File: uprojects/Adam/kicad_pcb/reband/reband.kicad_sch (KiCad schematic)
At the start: 3 parts, among them U1 ESP32-C3FH4, U2 LMV324MT, U3 MAX30009ENA+T

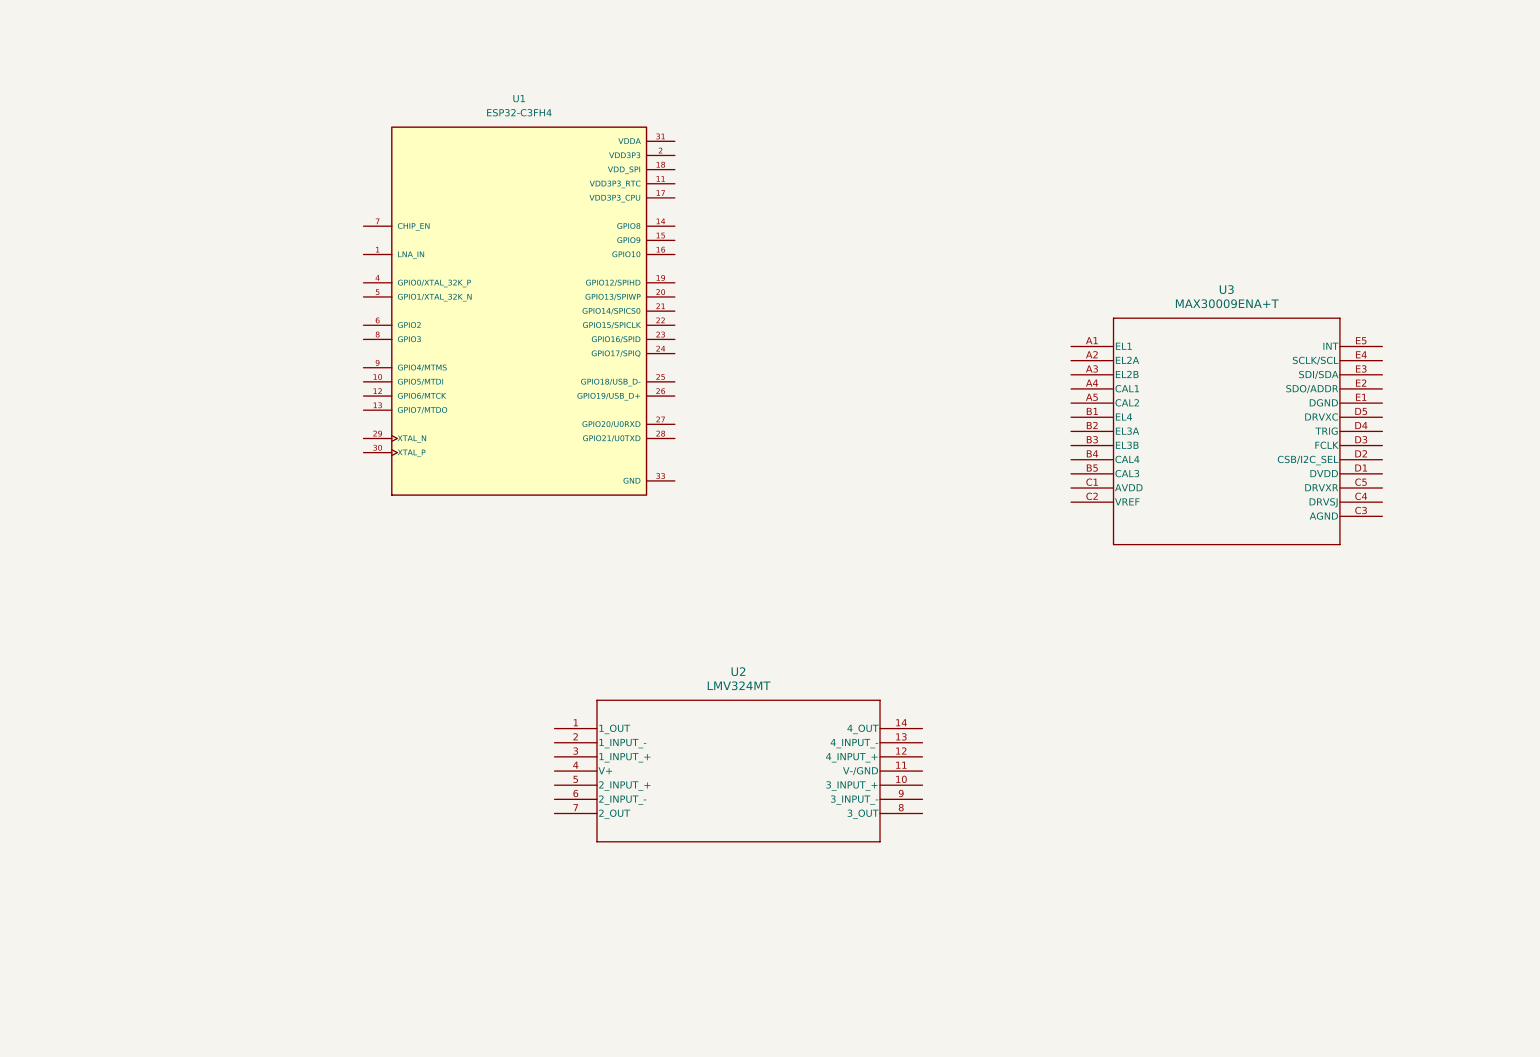
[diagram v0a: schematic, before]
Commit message: ROOM 25 MAY 2026 Updates
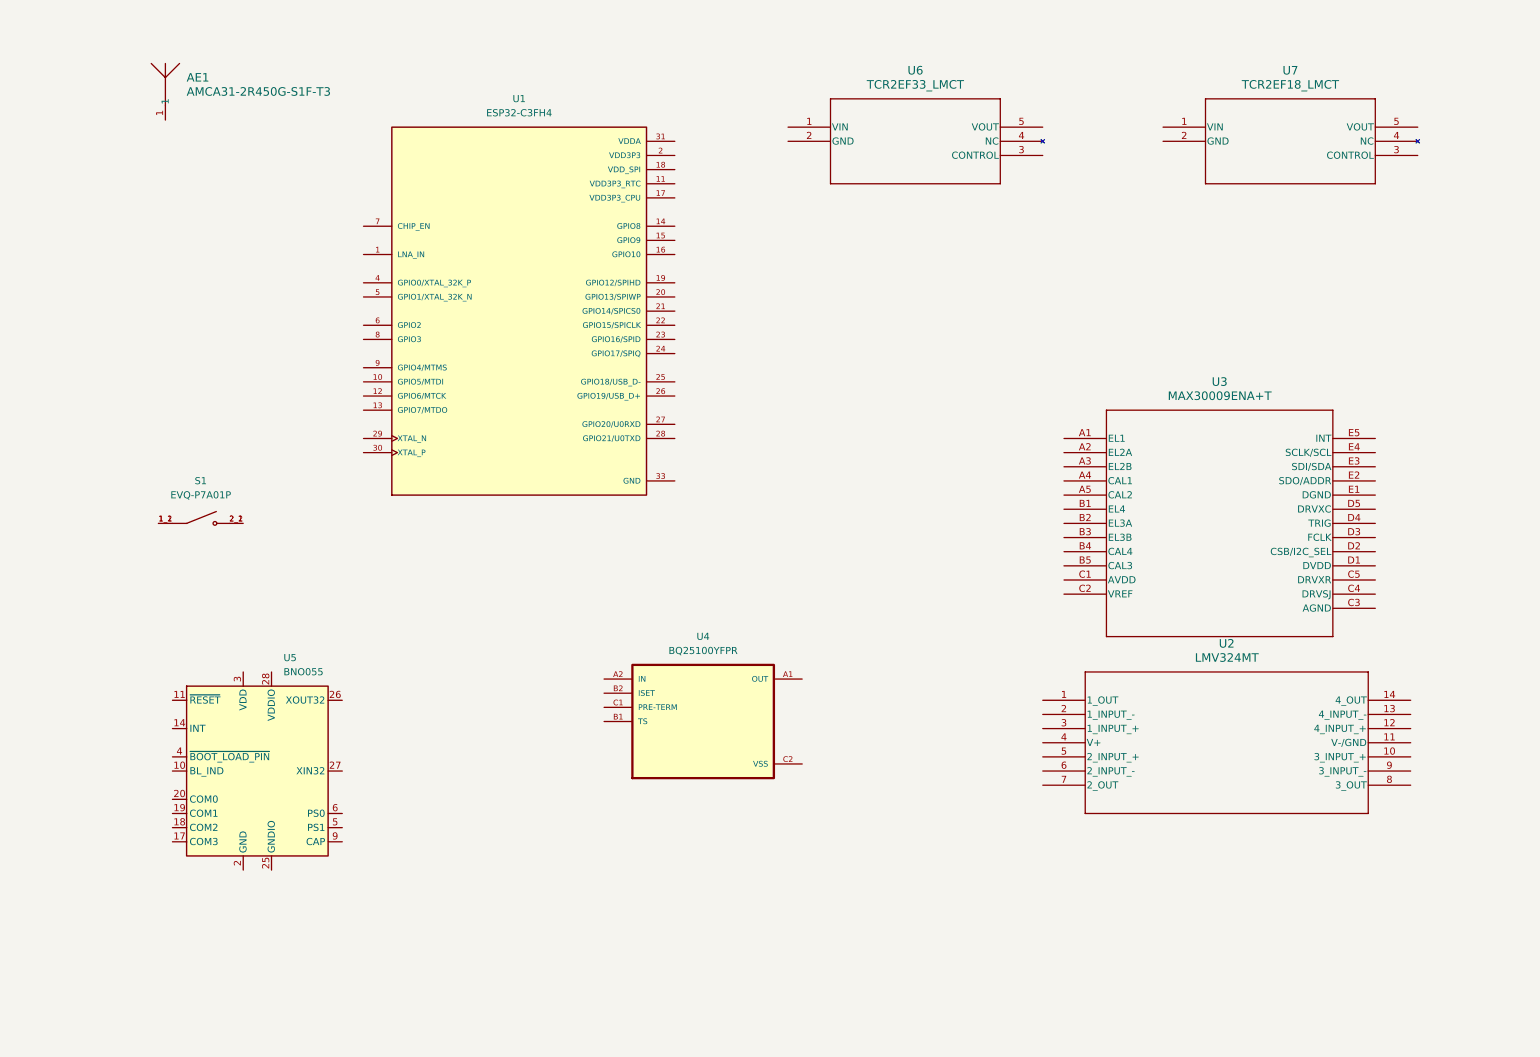
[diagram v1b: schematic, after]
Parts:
- added AE1: AMCA31-2R450G-S1F-T3, AMCA31_2R450G_S1F_T3:ANT_AMCA31-2R450G-S1F-T3_ABR, symbol AMCA31_2R450G_S1F_T3:AMCA31-2R450G-S1F-T3
- added S1: EVQ-P7A01P, EVQ_P7A01P:SW_EVQ-P7A01P, symbol EVQ-P7A01P:EVQ-P7A01P
- added U4: BQ25100YFPR, BQ25100YFPR:BGA6N40P3X2_157X88X50N, symbol BQ25100YFPR:BQ25100YFPR
- added U5: BNO055, Package_LGA:LGA-28_5.2x3.8mm_P0.5mm, symbol Sensor_Motion:BNO055
- added U6: TCR2EF33_LMCT, SOT-25 SMV_TOS, symbol TCR2EF33_LM_CT:TCR2EF33_LMCT
- added U7: TCR2EF18_LMCT, SOT-25 SMV_TOS, symbol TCR2EF18_LM_CT:TCR2EF18_LMCT
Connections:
- new net: S1.1_1, S1.1_2
- new net: S1.2_1, S1.2_2
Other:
- moved on the sheet: U2, U3

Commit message: Update 26 May 2026
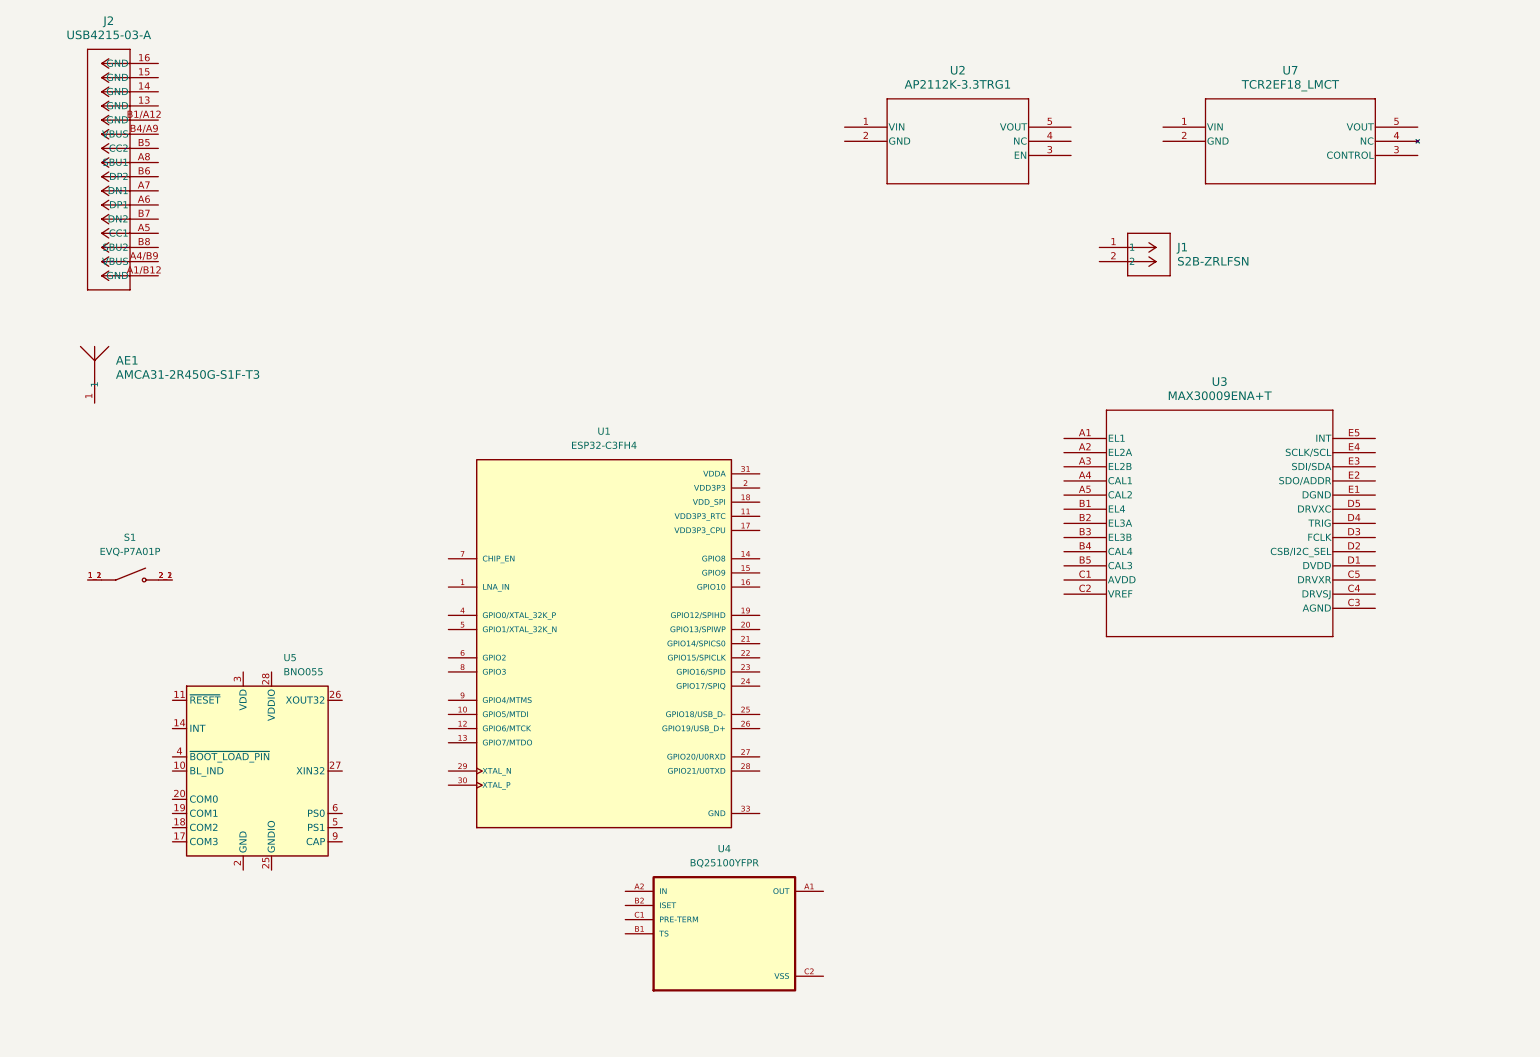
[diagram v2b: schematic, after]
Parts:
- removed U2: LMV324MT, LMV324MT:MTC14_TEX, symbol LMV324MT:LMV324MT
- removed U6: TCR2EF33_LMCT, SOT-25 SMV_TOS, symbol TCR2EF33_LM_CT:TCR2EF33_LMCT
- added J1: S2B-ZRLFSN, S2B_ZR_LF_SN:CONN_S2B-ZR_JST, symbol S2B_ZR_LF_SN:S2B-ZRLFSN
- added J2: USB4215-03-A, USB4215_03_A:CONN_8p94X6p5X3p16_12L_GCC, symbol USB4215_03_A:USB4215-03-A
- added U2: AP2112K-3.3TRG1, AP2112K_3_3TRG1:SOT_RG1_DIO, symbol AP2112K_3_3TRG1:AP2112K-3.3TRG1
- U7: footprint SOT-25 SMV_TOS -> TCR2EF18_LM_CT:SOT-25 SMV_TOS
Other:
- moved on the sheet: AE1, S1, U1, U4

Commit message: Update 28 May 2026
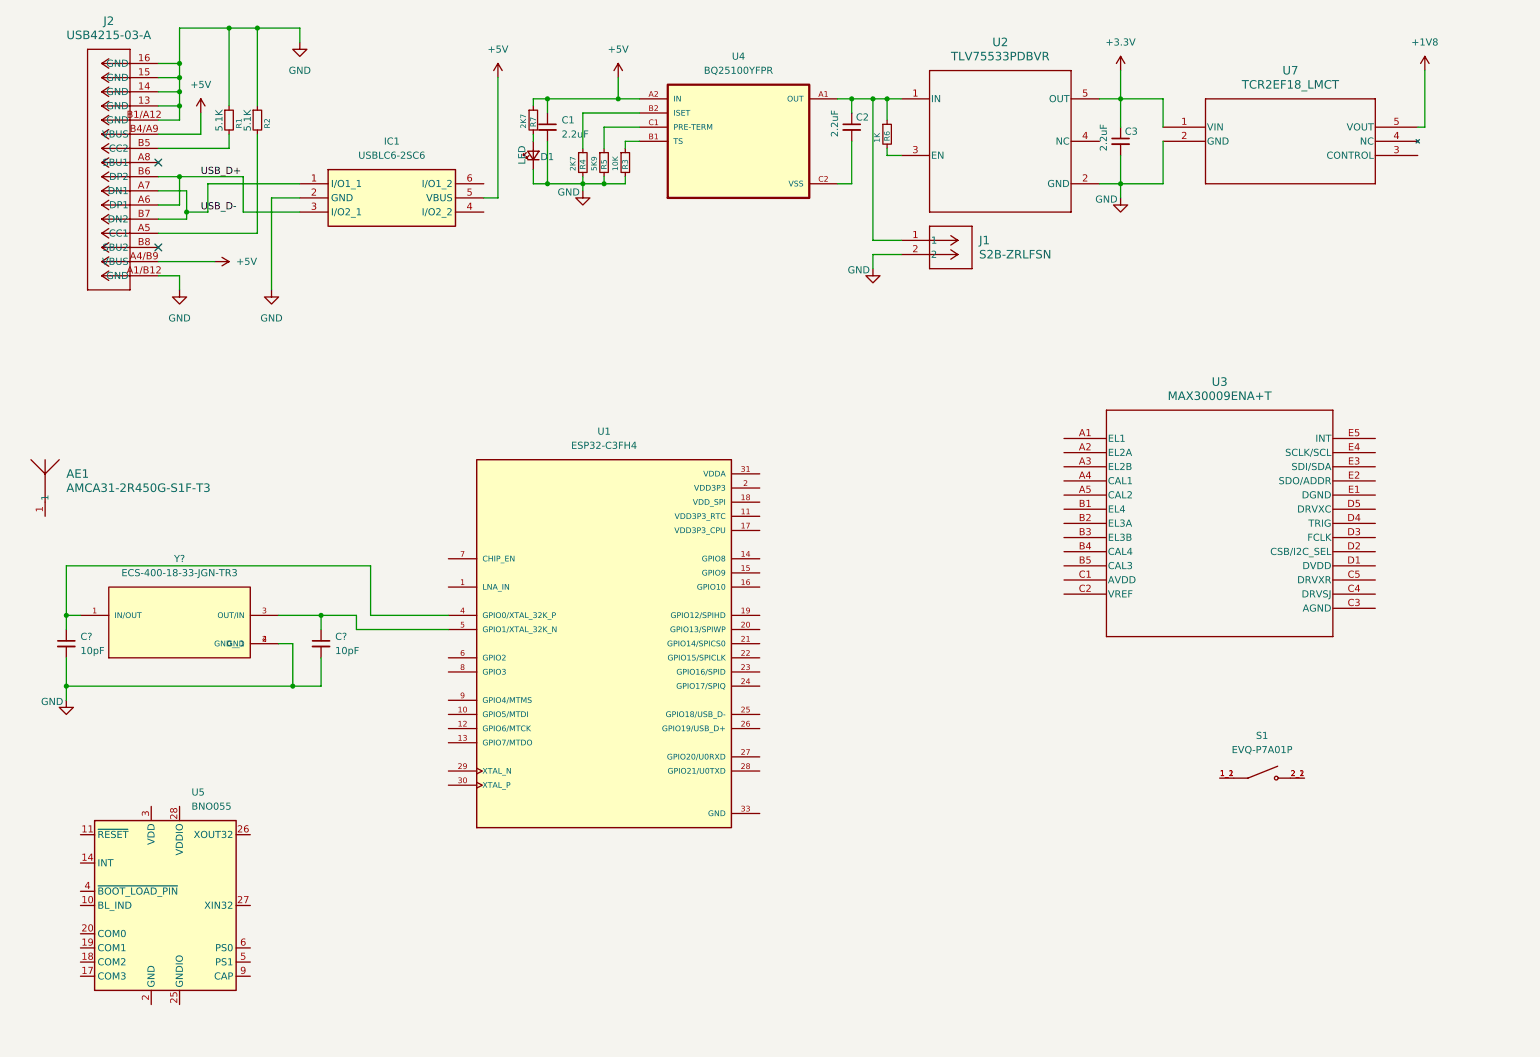
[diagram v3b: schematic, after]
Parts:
- removed U2: AP2112K-3.3TRG1, AP2112K_3_3TRG1:SOT_RG1_DIO, symbol AP2112K_3_3TRG1:AP2112K-3.3TRG1
- added C1, C2, C3: 2.2uF, Capacitor_SMD:C_0402_1005Metric_Pad0.74x0.62mm_HandSolder, symbol Device:C_Small
- added C? (x2): 10pF, Capacitor_SMD:C_0402_1005Metric_Pad0.74x0.62mm_HandSolder, symbol Device:C_Small
- added D1: LED, LED_SMD:LED_0402_1005Metric_Pad0.77x0.64mm_HandSolder, symbol Device:LED_Small
- added IC1: USBLC6-2SC6, USBLC6-2SC6:SOT95P280X145-6N, symbol USBLC6-2SC6:USBLC6-2SC6
- added R1, R2: 5.1K, Resistor_SMD:R_0402_1005Metric_Pad0.72x0.64mm_HandSolder, symbol Device:R_Small
- added R3: 10K, Resistor_SMD:R_0402_1005Metric_Pad0.72x0.64mm_HandSolder, symbol Device:R_Small
- added R4, R7: 2K7, Resistor_SMD:R_0402_1005Metric_Pad0.72x0.64mm_HandSolder, symbol Device:R_Small
- added R5: 5K9, Resistor_SMD:R_0402_1005Metric_Pad0.72x0.64mm_HandSolder, symbol Device:R_Small
- added R6: 1K, Resistor_SMD:R_0402_1005Metric_Pad0.72x0.64mm_HandSolder, symbol Device:R_Small
- added U2: TLV75533PDBVR, TLV75533PDBVR:DBV0005A_N, symbol TLV75533PDBVR:TLV75533PDBVR
- added Y?: ECS-400-18-33-JGN-TR3, ECS-400-18-33-JGN-TR3:XTAL_ECS-400-18-33-JGN-TR3, symbol ECS-400-18-33-JGN-TR3:ECS-400-18-33-JGN-TR3
- J1: DigiKey (none) -> 455-1669-ND; Manufacturer_Part_Number (none) -> S2B-ZR
- J2: DigiKey (none) -> 2073-USB4215-03-ATR-ND; Manufacturer_Part_Number (none) -> USB4215-03-A
- U4: DigiKey (none) -> 296-39931-2-ND; Manufacturer_Part_Number (none) -> BQ25100YFPR
- U7: DigiKey (none) -> TCR2EF18LM(CTTR-ND; Manufacturer_Part_Number (none) -> TCR2EF18,LM(CT
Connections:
- net at U4.A1 (OUT): now also J1.1, C2.1, R6.1, U2.1 (IN)
- net +5V: now reaches U4.A2 (IN)
- net +5V: now also J2.A4/B9 (VBUS), J2.B4/A9 (VBUS), C1.1, IC1.5 (VBUS), R7.1
- net at U4.B1 (TS): now also R3.1
- net at U4.B2 (ISET): now also R4.1
- net at U4.C1 (PRE-TERM): now also R5.1
- net at U4.C2 (VSS): now also C2.2
- net +3.3V: now reaches U7.1 (VIN)
- net +3.3V: now also C3.1, U2.5 (OUT)
- net GND: now reaches U7.2 (GND)
- net GND: now also J1.2, J2.13 (GND), J2.14 (GND), J2.15 (GND), J2.16 (GND), J2.A1/B12 (GND), J2.B1/A12 (GND), C1.2, C3.2, C?.2, C?.2, D1.1 (K), IC1.2 (GND), R1.1, R2.1, R3.2, R4.2, R5.2, U2.2 (GND), Y?.2 (GND), Y?.4 (GND__1)
- net +1V8: now reaches U7.5 (VOUT)
- net at U1.4 (GPIO0/XTAL_32K_P): now also C?.1, Y?.1 (IN/OUT)
- net at U1.5 (GPIO1/XTAL_32K_N): now also C?.1, Y?.3 (OUT/IN)
- net at J2.A5 (CC1): now also R2.2
- net USB_D+: now reaches J2.A6 (DP1)
- net USB_D+: now also J2.B6 (DP2), IC1.3 (I/O2_1)
- net USB_D-: now reaches J2.A7 (DN1)
- net USB_D-: now also J2.B7 (DN2), IC1.1 (I/O1_1)
- net at J2.B5 (CC2): now also R1.2
- new net: R6.2, U2.3 (EN)
- new net: D1.2 (A), R7.2
- no-connect marks 0 -> 2
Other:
- moved on the sheet: AE1, J1, S1, U4, U5

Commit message: Update 28 May 2026
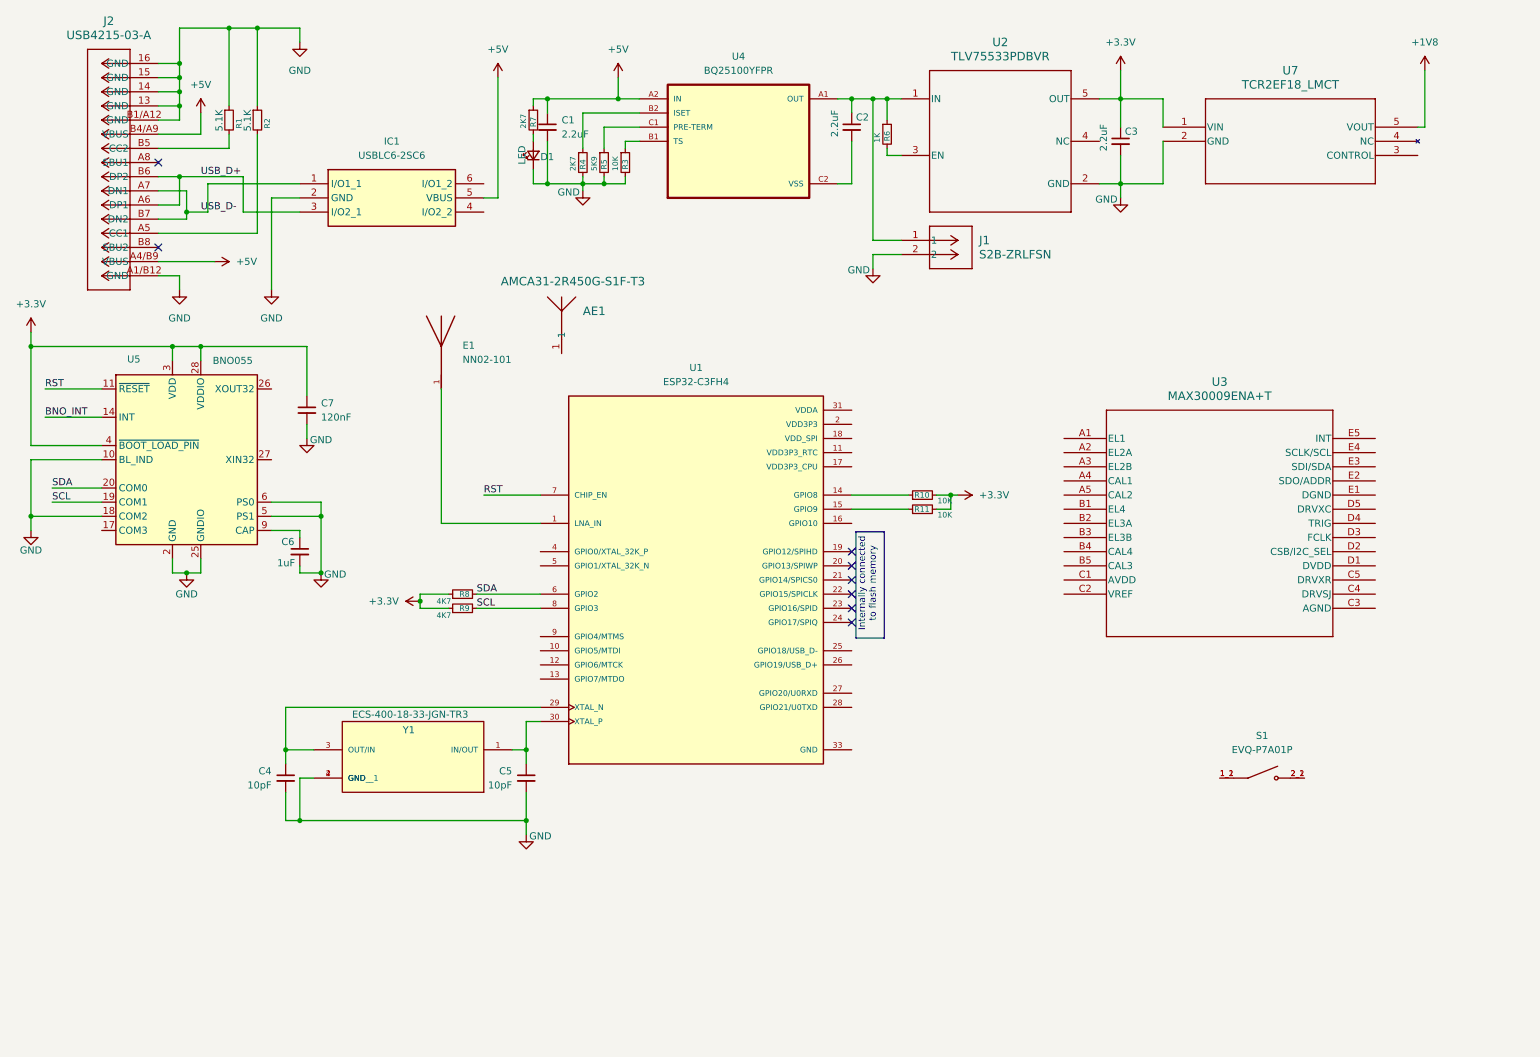
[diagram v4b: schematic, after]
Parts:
- added C6: 1uF, Capacitor_SMD:C_0402_1005Metric_Pad0.74x0.62mm_HandSolder, symbol Device:C_Small
- added C7: 120nF, Capacitor_SMD:C_0402_1005Metric_Pad0.74x0.62mm_HandSolder, symbol Device:C_Small
- added E1: NN02-101, NN02_101:XCVR_NN02-101, symbol NN02-101:NN02-101
- added R10, R11: 10K, Resistor_SMD:R_0402_1005Metric_Pad0.72x0.64mm_HandSolder, symbol Device:R_Small
- added R8, R9: 4K7, Resistor_SMD:R_0402_1005Metric_Pad0.72x0.64mm_HandSolder, symbol Device:R_Small
- Y1: renamed from Y?; footprint ECS-400-18-33-JGN-TR3:XTAL_ECS-400-18-33-JGN-TR3 -> ECS_400_18_33_JGN_TR3:XTAL_ECS-400-18-33-JGN-TR3
- gave numbers to parts that had none: 2
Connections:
- net +3.3V: now also U5.28 (VDDIO), U5.3 (VDD), U5.4 (~{BOOT_LOAD_PIN}), C7.1, R10.2, R11.2, R8.1, R9.1
- net GND: now also U5.10 (BL_IND), U5.18 (COM2), U5.2 (GND), U5.25 (GNDIO), U5.5 (PS1), U5.6 (PS0), C6.2, C7.2
- net at C4.1, Y1.3 (OUT/IN): now also U1.29 (XTAL_N); no longer U1.5 (GPIO1/XTAL_32K_N)
- net RST: now reaches U5.11 (~{RESET})
- net RST: now also U1.7 (CHIP_EN)
- net BNO_INT: now reaches U5.14 (INT)
- net SCL: now reaches U5.19 (COM1)
- net SCL: now also U1.8 (GPIO3), R9.2
- net SDA: now reaches U5.20 (COM0)
- net SDA: now also U1.6 (GPIO2), R8.2
- net at U5.9 (CAP): now also C6.1
- net at C5.1, Y1.1 (IN/OUT): now also U1.30 (XTAL_P); no longer U1.4 (GPIO0/XTAL_32K_P)
- net at U1.1 (LNA_IN): now also E1.1
- net at U1.14 (GPIO8): now also R10.1
- net at U1.15 (GPIO9): now also R11.1
- no-connect marks 2 -> 8
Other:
- note added: "Internally connected to flash memory"
- moved on the sheet: AE1, C4, C5, U1, U5, Y1
